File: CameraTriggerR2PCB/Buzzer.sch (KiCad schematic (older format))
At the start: 1 part

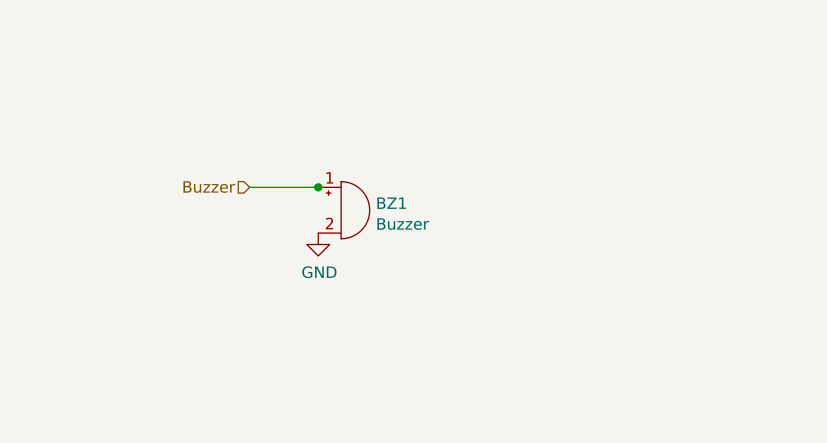
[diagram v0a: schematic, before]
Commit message: Add files via upload
First cut at modules
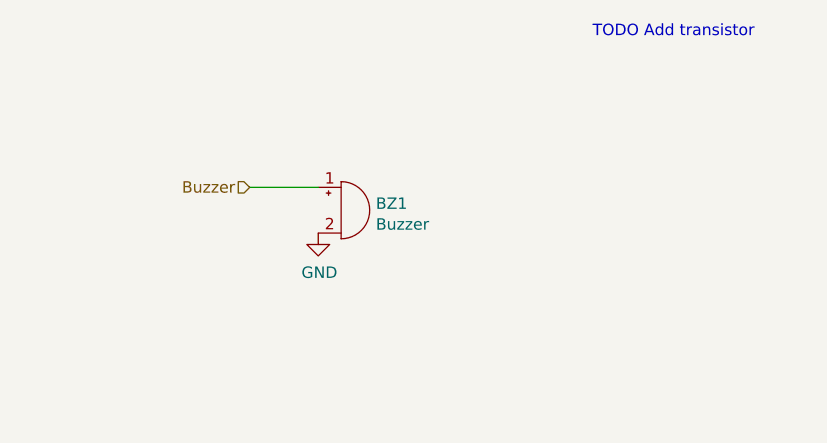
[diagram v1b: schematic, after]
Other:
- note added: "TODO Add transistor"
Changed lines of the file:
@@
 $Descr A4 11693 8268
 encoding utf-8
-Sheet 8 8
+Sheet 6 9
 Title ""
 Date ""
@@
 Text HLabel 1550 3750 0    50   Input ~ 0
 Buzzer
-Connection ~ 1850 3750
+Text Notes 3050 3100 0    50   ~ 0
+TODO Add transistor
 $EndSCHEMATC

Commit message: Add files via upload
Changes from 5/17 Zoom sensor
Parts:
- added Q4: 2N2219, Package_TO_SOT_THT:TO-39-3, symbol Transistor_BJT:2N2219
- added R11, R12: R, symbol Device:R
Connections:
- net labels added: +3.3V
- wire segments 1 -> 8
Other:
- note removed: "TODO Add transistor"
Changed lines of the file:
@@
 Comment4 ""
 $EndDescr
-Wire Wire Line
-	1550 3750 1850 3750
+Text HLabel 900  3750 0    50   Input ~ 0
+Buzzer
 $Comp
-L power:GND #PWR?
-U 1 1 5ECC7811
-P 1850 3950
-AR Path="/5ECC7811" Ref="#PWR?"  Part="1"
-AR Path="/5ECC61B0/5ECC7811" Ref="#PWR044"  Part="1"
-F 0 "#PWR044" H 1850 3700 50  0001 C CNN
-F 1 "GND" H 1855 3777 50  0000 C CNN
-F 2 "" H 1850 3950 50  0001 C CNN
-F 3 "" H 1850 3950 50  0001 C CNN
-	1    1850 3950
+L Device:R R12
+U 1 1 5EC38A74
+P 1600 3850
+F 0 "R12" H 1670 3896 50  0000 L CNN
+F 1 "R" H 1670 3805 50  0000 L CNN
+F 2 "" V 1530 3850 50  0001 C CNN
+F 3 "~" H 1600 3850 50  0001 C CNN
+	1    1600 3850
 	1    0    0    -1
 $EndComp
+Wire Wire Line
+	1600 3700 1750 3700
+Wire Wire Line
+	1850 3700 1850 3750
 $Comp
 L Device:Buzzer BZ?
@@
 	1    0    0    -1
 $EndComp
-Text HLabel 1550 3750 0    50   Input ~ 0
-Buzzer
-Text Notes 3050 3100 0    50   ~ 0
-TODO Add transistor
+Wire Wire Line
+	1850 3950 1850 4000
+Wire Wire Line
+	1850 4000 1600 4000
+$Comp
+L power:+3.3V #PWR046
+U 1 1 5EC3BC3C
+P 1750 3700
+F 0 "#PWR046" H 1750 3550 50  0001 C CNN
+F 1 "+3.3V" H 1765 3873 50  0000 C CNN
+F 2 "" H 1750 3700 50  0001 C CNN
+F 3 "" H 1750 3700 50  0001 C CNN
+	1    1750 3700
+	1    0    0    -1
+$EndComp
+Connection ~ 1750 3700
+Wire Wire Line
+	1750 3700 1850 3700
+$Comp
+L Transistor_BJT:2N2219 Q4
+U 1 1 5EC3C5F5
+P 1500 4200
+F 0 "Q4" H 1690 4246 50  0000 L CNN
+F 1 "2N2219" H 1690 4155 50  0000 L CNN
+F 2 "Package_TO_SOT_THT:TO-39-3" H 1700 4125 50  0001 L CIN
+F 3 "http://www.onsemi.com/pub_link/Collateral/2N2219-D.PDF" H 1500 4200 50  0001 L CNN
+	1    1500 4200
+	1    0    0    -1
+$EndComp
+Connection ~ 1600 4000
+$Comp
+L power:GND #PWR045
+U 1 1 5EC3D80C
+P 1600 4450
+F 0 "#PWR045" H 1600 4200 50  0001 C CNN
+F 1 "GND" H 1605 4277 50  0000 C CNN
+F 2 "" H 1600 4450 50  0001 C CNN
+F 3 "" H 1600 4450 50  0001 C CNN
+	1    1600 4450
+	1    0    0    -1
+$EndComp
+$Comp
+L Device:R R11
+U 1 1 5EC3DB81
+P 1300 4050
+F 0 "R11" H 1370 4096 50  0000 L CNN
+F 1 "R" H 1370 4005 50  0000 L CNN
+F 2 "" V 1230 4050 50  0001 C CNN
+F 3 "~" H 1300 4050 50  0001 C CNN
+	1    1300 4050
+	1    0    0    -1
+$EndComp
+Wire Wire Line
+	1600 4400 1600 4450
+Wire Wire Line
+	1300 3900 1300 3750
+Wire Wire Line
+	1300 3750 900  3750
+Connection ~ 1600 4400
+Connection ~ 1600 4450
 $EndSCHEMATC
